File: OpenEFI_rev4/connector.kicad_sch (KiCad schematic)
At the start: 58 parts, among them J6 1241434-1, Q10 PMN30XPX, Q20 PMN30XPX, Q5 SS8050, Q6 IRLZ44N, Q7 IRLZ44N, U14 MIC5205-3.3YM5, U16 TPS5430DDA, U17 L78M05ABDT-TR, U4 AMS1117-3.3, U6 LT4363IMS

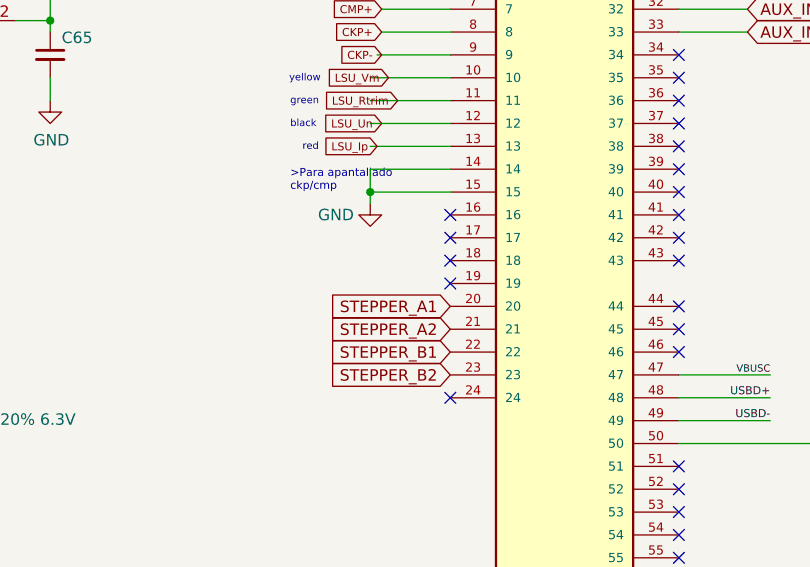
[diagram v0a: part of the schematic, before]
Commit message: wip SD card
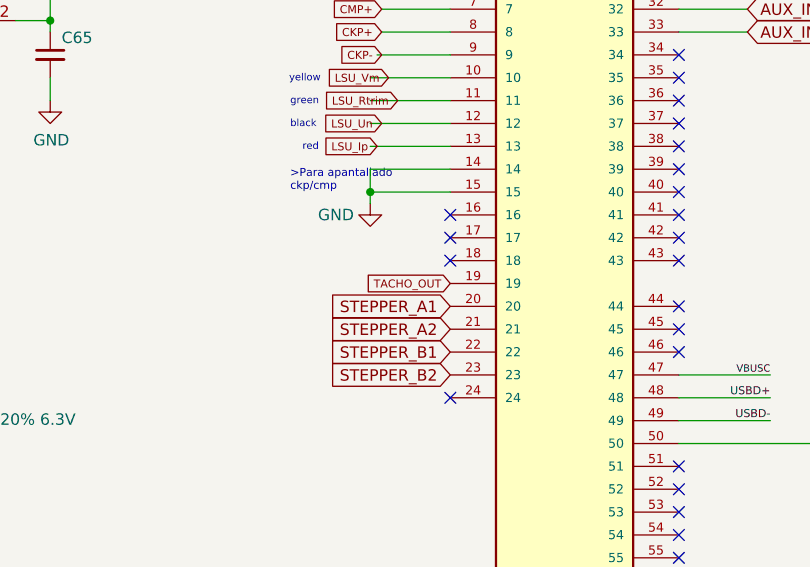
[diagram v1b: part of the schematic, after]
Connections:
- net TACHO_OUT: now reaches J6.19
- no-connect marks 32 -> 31
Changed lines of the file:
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@@
   (no_connect (at 91.44 163.83))
   (no_connect (at 172.72 101.6))
-  (no_connect (at 147.32 76.2))
   (no_connect (at 172.72 55.88))
   (wire (pts (xy 222.25 58.42) (xy 231.14 58.42))
@@
     )
   )
+  (global_label "TACHO_OUT" (shape input) (at 147.32 76.2 180)
+    (effects (font (size 0.889 0.889)) (justify right))
+    (property "Intersheetrefs" "${INTERSHEET_REFS}" (at 144.0223 76.2555 0)
+      (effects (font (size 0.889 0.889)) (justify right) hide)
+    )
+  )

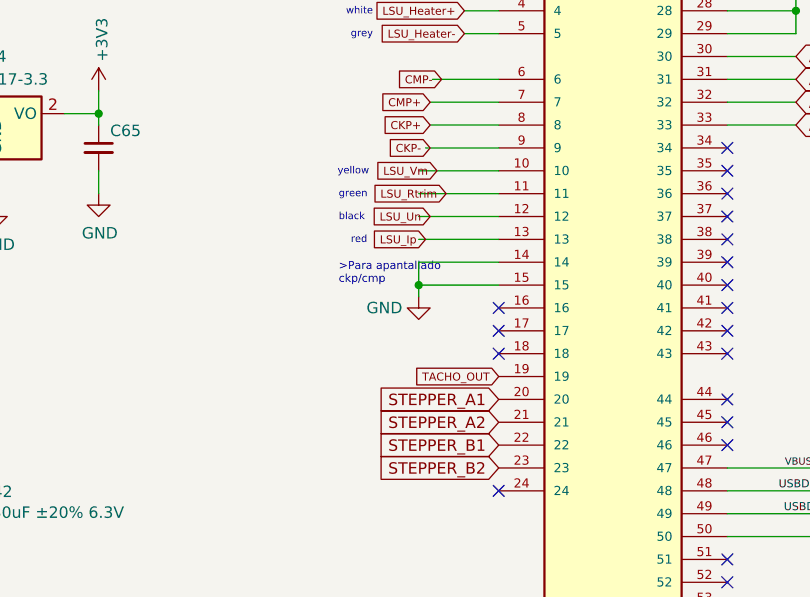
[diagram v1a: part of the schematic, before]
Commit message: WIP Rev4 SPI
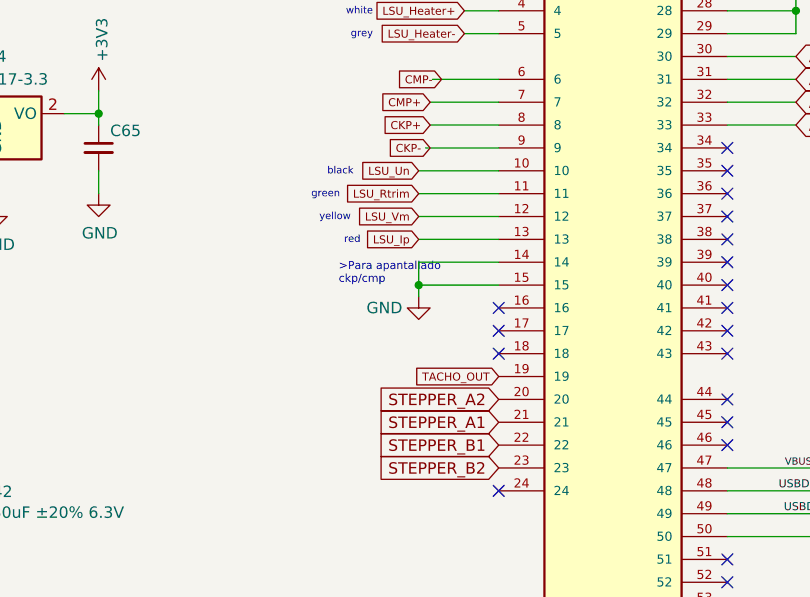
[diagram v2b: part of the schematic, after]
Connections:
- net LSU_Un: now also J6.10; no longer J6.12
- net LSU_Vm: now also J6.12; no longer J6.10
- net STEPPER_A1: now also J6.21; no longer J6.20
- net STEPPER_A2: now also J6.20; no longer J6.21
